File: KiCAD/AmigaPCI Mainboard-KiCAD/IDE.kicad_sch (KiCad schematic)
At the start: 43 parts, among them CN20 SECONDARY IDE, CN227 JTAG/SWD, CN5 PRIMARY IDE, CN6 IDE_LED, J202 SYSTEM CLK, J905 CABLE SELECT, U2 XC9572XL-VQ64, U220 74AHCT08, U900 74HCT245, U901 74HCT245, U902 74HCT245, U904 74HCT245, U905 74FCT646, U906 74FCT646

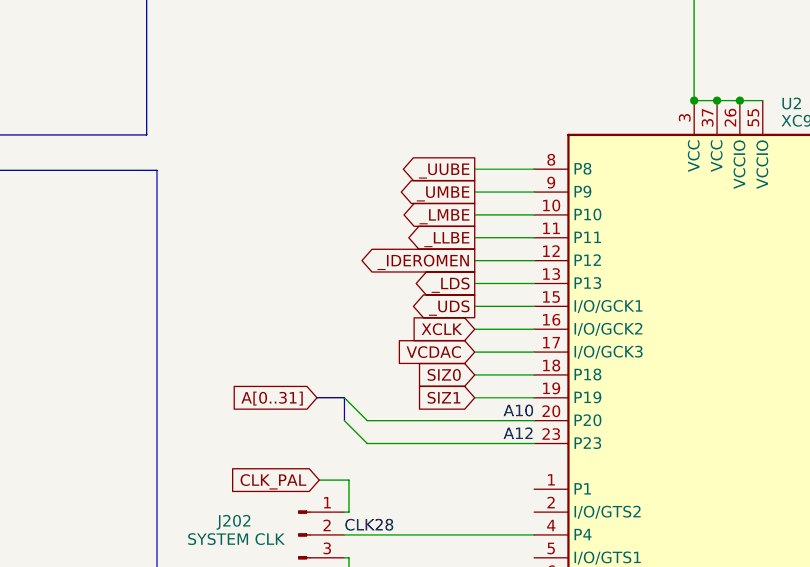
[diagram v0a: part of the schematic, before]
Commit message: Schematic and Routing 14-DEC-2023
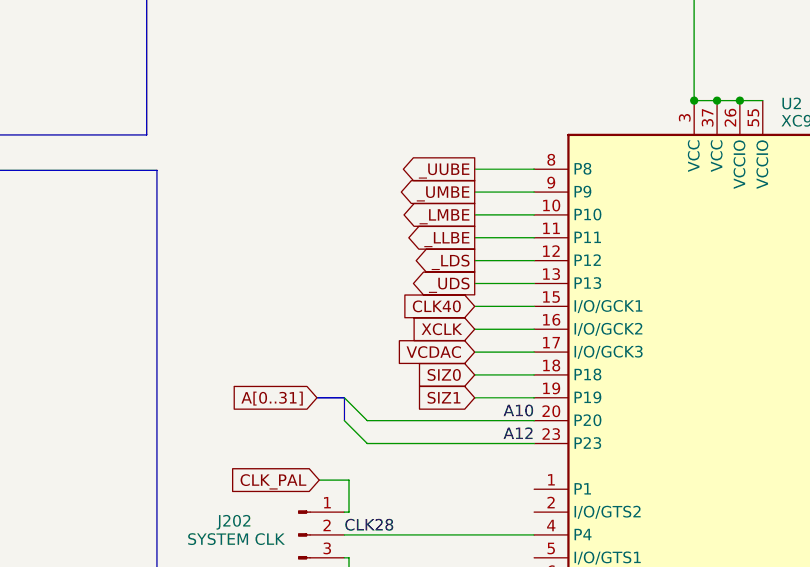
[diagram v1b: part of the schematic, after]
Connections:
- net _IDEROMEN is gone; now on net _LDS: U2.12 (P12)
- net _LDS: no longer U2.13 (P13)
- net _UDS: now also U2.13 (P13); no longer U2.15 (I/O/GCK1)
- new net CLK40: U2.15 (I/O/GCK1)
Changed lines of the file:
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@@
-    )
-  )
-  (global_label "_IDEROMEN" (shape output) (at 234.696 168.148 180) (fields_autoplaced)
-    (effects (font (size 1.27 1.27)) (justify right))
-    (property "Intersheetrefs" "${INTERSHEET_REFS}" (at 221.2674 168.148 0)
-      (effects (font (size 1.27 1.27)) (justify right))
     )
   )
@@
     (property "Intersheetrefs" "${INTERSHEET_REFS}" (at 297.449 188.468 0)
       (effects (font (size 1.27 1.27)) (justify left))
+    )
+  )
+  (global_label "CLK40" (shape input) (at 234.696 173.228 180) (fields_autoplaced)
+    (effects (font (size 1.27 1.27)) (justify right))
+    (property "Intersheetrefs" "${INTERSHEET_REFS}" (at 225.7237 173.228 0)
+      (effects (font (size 1.27 1.27)) (justify right))
     )
   )
@@
     )
   )
-  (global_label "_LDS" (shape output) (at 234.696 170.688 180) (fields_autoplaced)
+  (global_label "_LDS" (shape output) (at 234.696 168.148 180) (fields_autoplaced)
     (effects (font (size 1.27 1.27)) (justify right))
-    (property "Intersheetrefs" "${INTERSHEET_REFS}" (at 227.315 170.688 0)
+    (property "Intersheetrefs" "${INTERSHEET_REFS}" (at 227.315 168.148 0)
       (effects (font (size 1.27 1.27)) (justify right))
     )
@@
     )
   )
-  (global_label "_UDS" (shape output) (at 234.696 173.228 180) (fields_autoplaced)
+  (global_label "_UDS" (shape output) (at 234.696 170.688 180) (fields_autoplaced)
     (effects (font (size 1.27 1.27)) (justify right))
-    (property "Intersheetrefs" "${INTERSHEET_REFS}" (at 227.0126 173.228 0)
+    (property "Intersheetrefs" "${INTERSHEET_REFS}" (at 227.0126 170.688 0)
       (effects (font (size 1.27 1.27)) (justify right))
     )

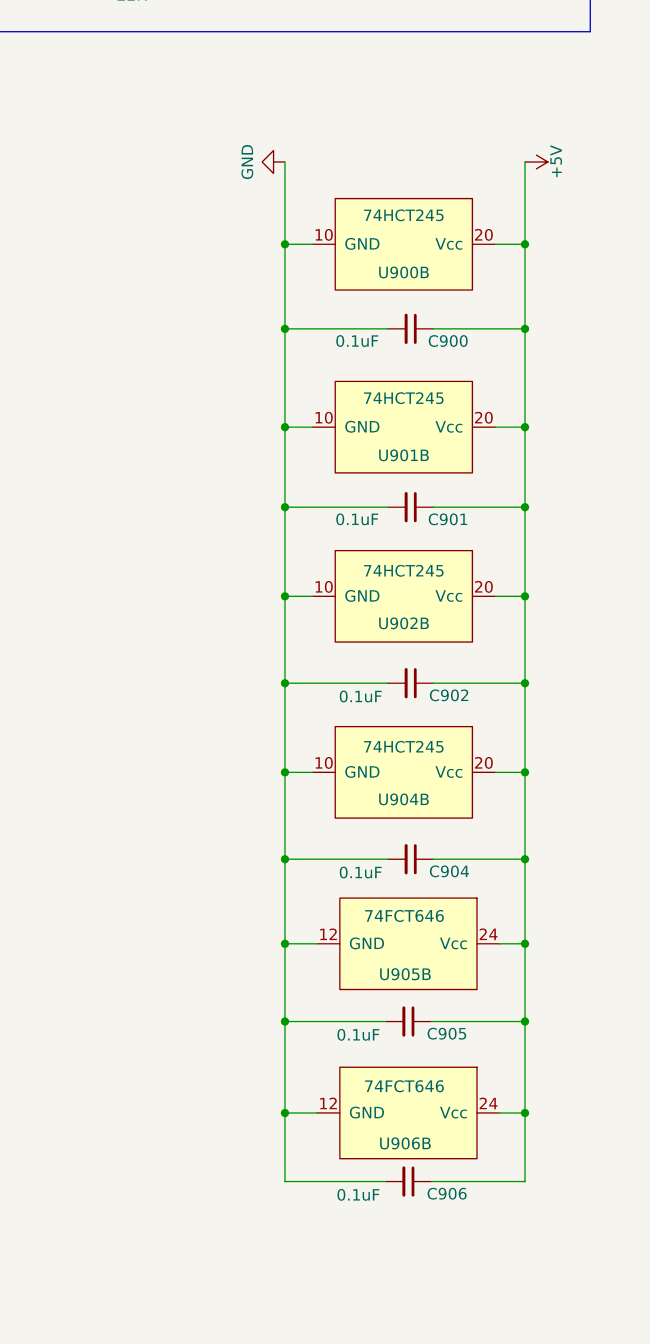
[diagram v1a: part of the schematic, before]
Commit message: Schematic Cleanup 15-DEC-2023
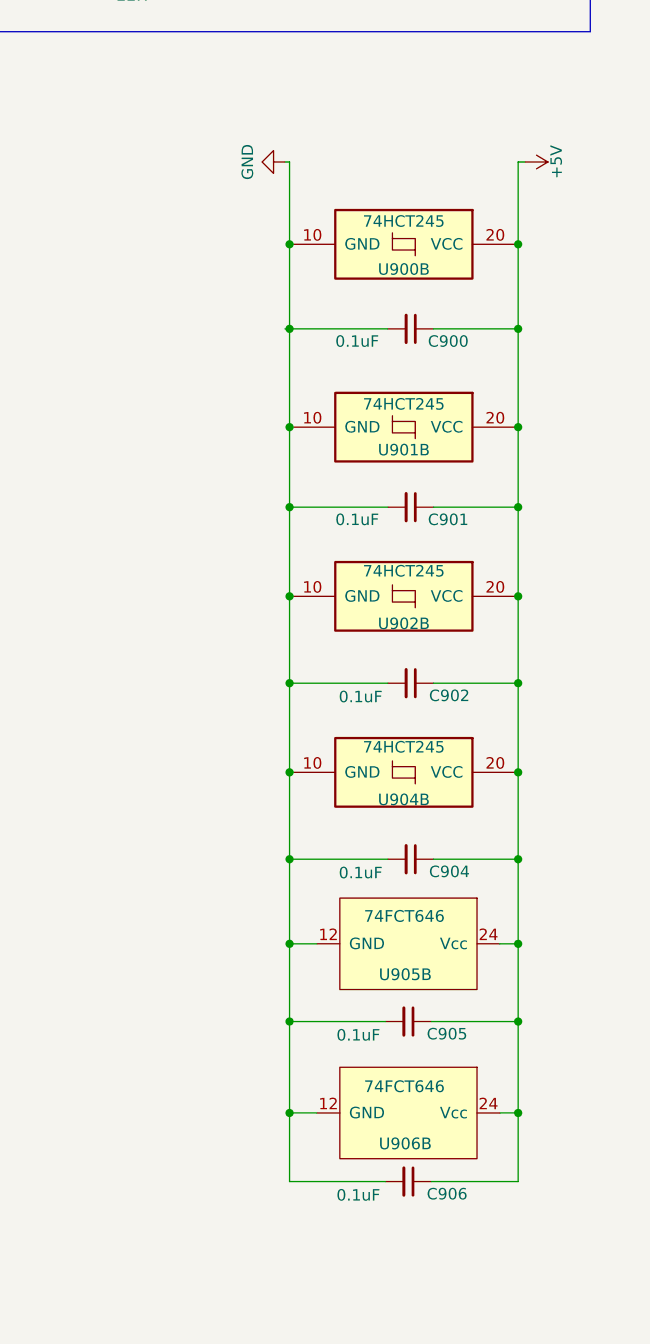
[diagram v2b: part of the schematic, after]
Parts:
- CN20, CN5: symbol Connector_Generic:Conn_02x20_Odd_Even -> AmigaPCI-Symbols:Conn_02x20_IDE
- U900, U901, U902, U904: symbol N2630:74HCT245 -> AmigaPCI-Symbols:74LVC245

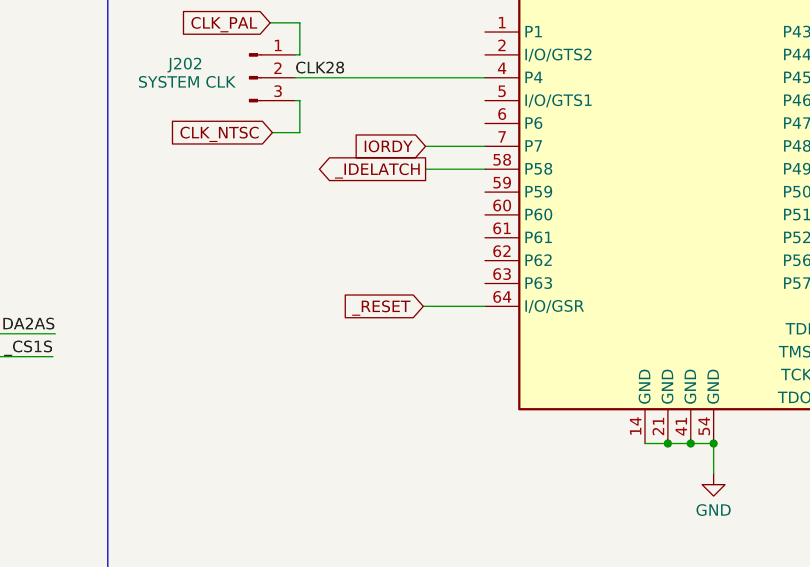
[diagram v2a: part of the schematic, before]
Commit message: Routing 17-DEC-2023
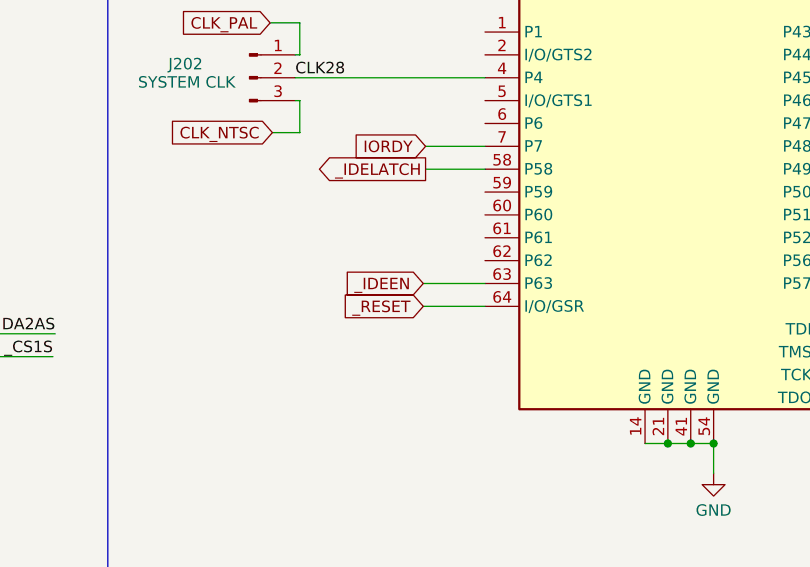
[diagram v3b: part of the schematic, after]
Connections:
- net _IDEEN: now reaches U2.63 (P63)
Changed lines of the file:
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@@
+    (stroke (width 0) (type default))
+  )
+  (wire (pts (xy 234.442 221.488) (xy 241.3 221.488))
     (stroke (width 0) (type default))
   )
@@
       (effects (font (size 1.27 1.27)) (justify right))
     )
+  )
+  (global_label "_IDEEN" (shape input) (at 234.442 221.488 180) (fields_autoplaced)
+    (effects (font (size 1.27 1.27)) (justify right))
+    (property "Intersheetrefs" "${INTERSHEET_REFS}" (at 224.9859 221.488 0)
+      (effects (font (size 1.27 1.27)) (justify right))
+    )

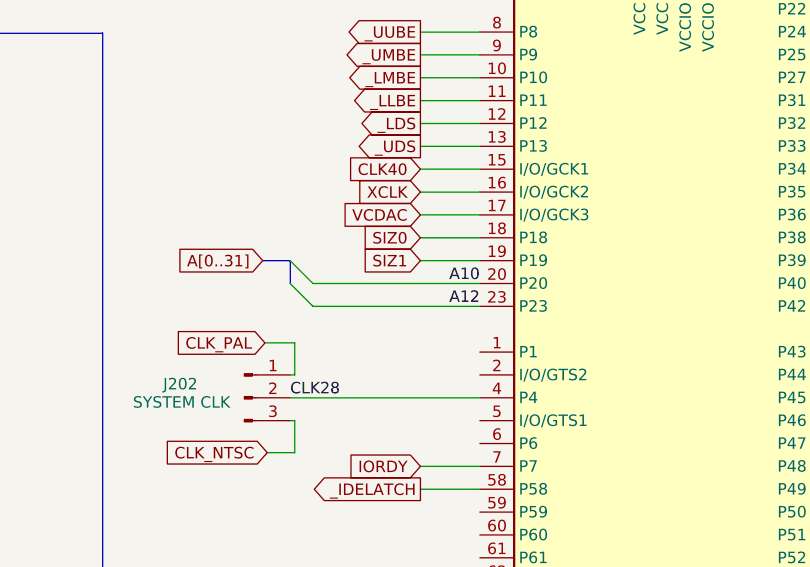
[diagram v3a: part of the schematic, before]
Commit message: Routing 19-DEC-2023
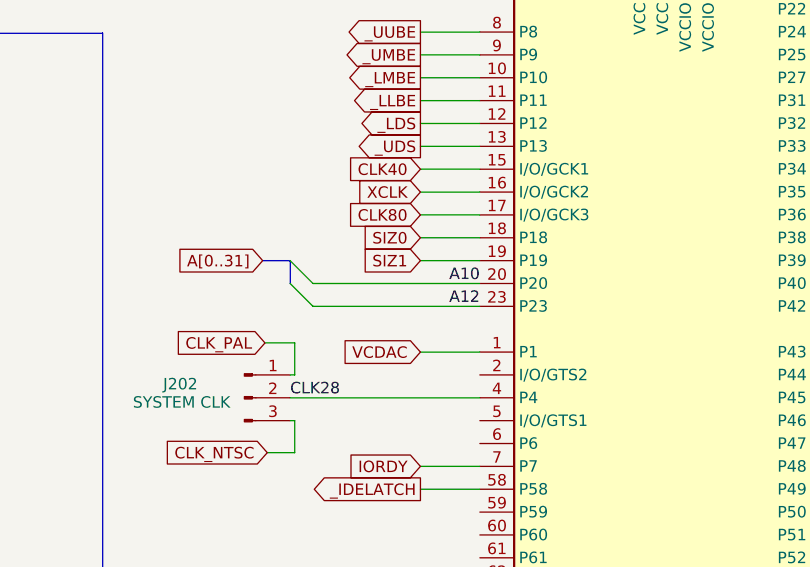
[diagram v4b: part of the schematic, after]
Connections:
- net VCDAC: now also U2.1 (P1); no longer U2.17 (I/O/GCK3)
- new net CLK80: U2.17 (I/O/GCK3)
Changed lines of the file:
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@@
+    (stroke (width 0) (type default))
+  )
+  (wire (pts (xy 234.696 193.548) (xy 241.3 193.548))
     (stroke (width 0) (type default))
   )
@@
     )
   )
-  (global_label "VCDAC" (shape input) (at 234.696 178.308 180) (fields_autoplaced)
+  (global_label "CLK80" (shape input) (at 234.696 178.308 180) (fields_autoplaced)
     (effects (font (size 1.27 1.27)) (justify right))
-    (property "Intersheetrefs" "${INTERSHEET_REFS}" (at 225.803 178.308 0)
+    (property "Intersheetrefs" "${INTERSHEET_REFS}" (at 225.7237 178.308 0)
       (effects (font (size 1.27 1.27)) (justify right))
     )
@@
     )
   )
+  (global_label "VCDAC" (shape input) (at 234.696 193.548 180) (fields_autoplaced)
+    (effects (font (size 1.27 1.27)) (justify right))
+    (property "Intersheetrefs" "${INTERSHEET_REFS}" (at 225.803 193.548 0)
+      (effects (font (size 1.27 1.27)) (justify right))
+    )
+  )

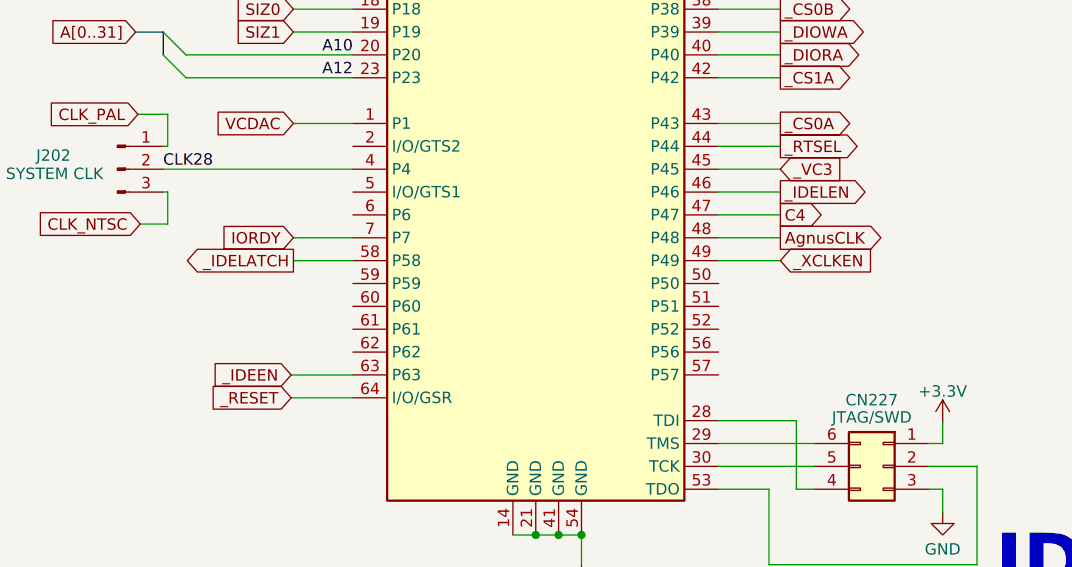
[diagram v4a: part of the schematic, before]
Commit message: Routing 21-DEC-2023
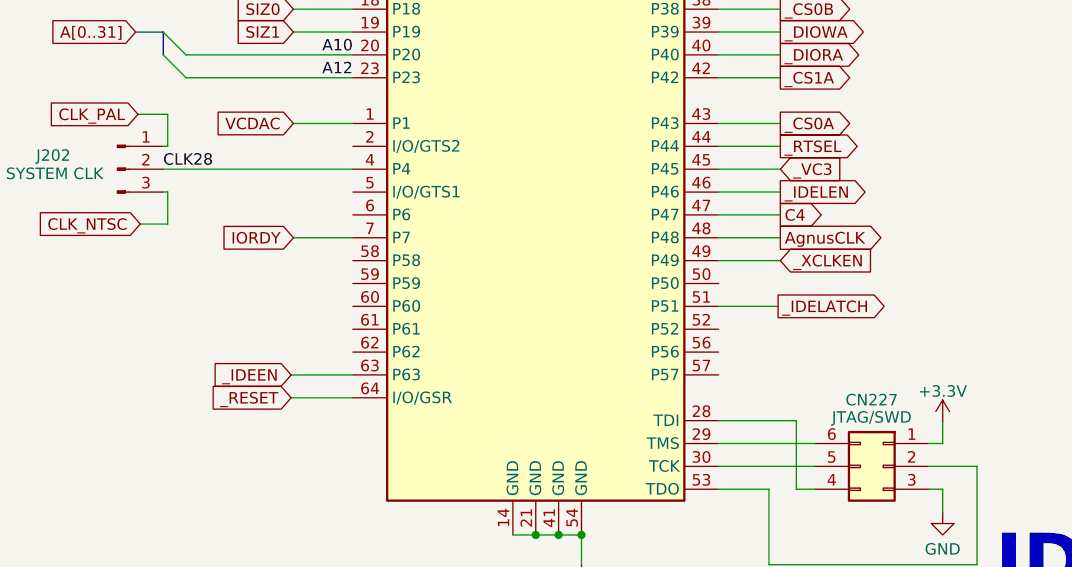
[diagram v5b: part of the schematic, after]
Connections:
- net _IDELATCH: now also U2.51 (P51); no longer U2.58 (P58)
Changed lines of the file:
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@@
     (stroke (width 0) (type default))
   )
-  (wire (pts (xy 234.696 208.788) (xy 241.3 208.788))
+  (wire (pts (xy 288.544 213.868) (xy 281.94 213.868))
     (stroke (width 0) (type default))
   )
@@
     )
   )
-  (global_label "_IDELATCH" (shape output) (at 234.696 208.788 180) (fields_autoplaced)
-    (effects (font (size 1.27 1.27)) (justify right))
-    (property "Intersheetrefs" "${INTERSHEET_REFS}" (at 222.114 208.788 0)
-      (effects (font (size 1.27 1.27)) (justify right))
-    )
-  )
+  (global_label "_IDELATCH" (shape output) (at 288.544 213.868 0) (fields_autoplaced)
+    (effects (font (size 1.27 1.27)) (justify left))
+    (property "Intersheetrefs" "${INTERSHEET_REFS}" (at 301.2054 213.868 0)
+      (effects (font (size 1.27 1.27)) (justify left))
+    )
+  )
